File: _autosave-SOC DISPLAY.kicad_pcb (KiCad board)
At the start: 2 copper layers, 44.7 x 50.3 mm, 87 parts, among them IC101 LM5164QDDATQ1, IC501 CM BLE, J201 PRG, J202 Conn_01x05_Socket, J203 OLED, J204 OLED, J205 Conn_01x02_Socket, J601 Conn_01x02_Pin, J602 Conn_01x02_Pin, Q301 NDT3055L, U101 TPS563200, U102 LP2985-3.3, U201 STM32G0B1CBTx, U202 MAX485E, U401 TJA1051T-3, U601 INA228AQDGSRQ1

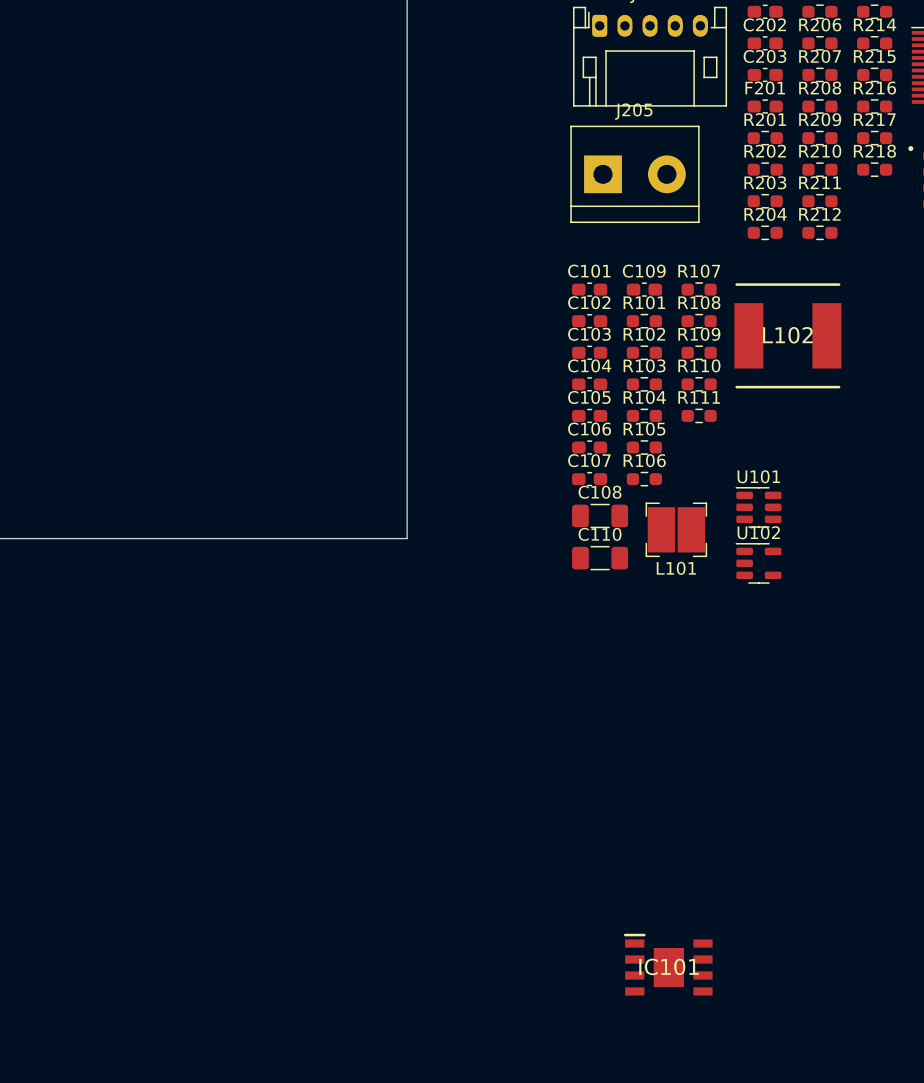
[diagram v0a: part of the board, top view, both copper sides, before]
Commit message: New
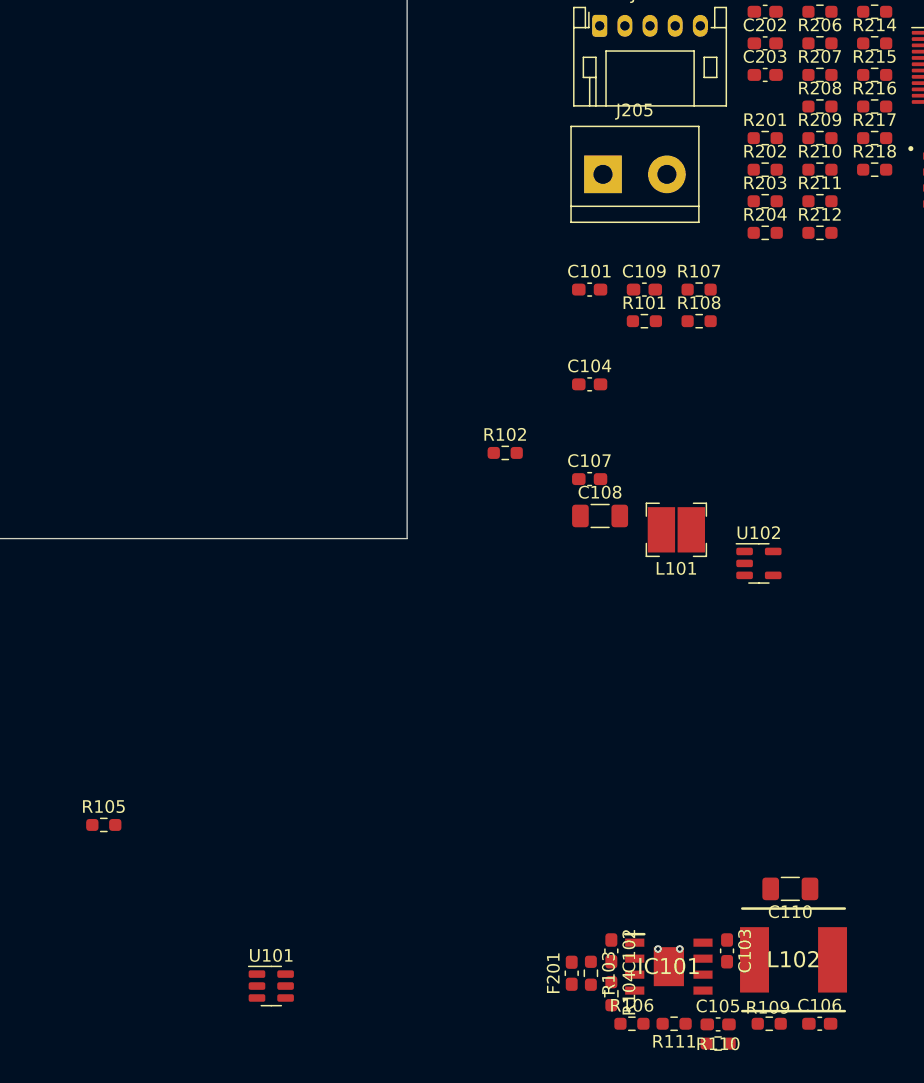
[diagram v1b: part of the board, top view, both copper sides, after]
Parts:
- C101: value 0.1uf -> 22uf
- moved F201 70.6 mm to (87.9, 117.9), turned to 90 degrees
- moved U101 54.3 mm to (64.0, 118.9)
- moved R109 53.6 mm to (103.6, 121.9)
- moved R110 52.4 mm to (99.5, 123.4), turned to 180 degrees
- moved R105 52.4 mm to (50.7, 106.1)
- moved C102 50.1 mm to (91.0, 116.1), turned to -90 degrees
- moved L102 49.6 mm to (105.5, 116.8)
- moved C105 49.4 mm to (99.5, 121.9)
- moved C106 49.3 mm to (107.6, 121.9)
- moved C103 48.8 mm to (100.2, 116.1), turned to -90 degrees
- moved R111 48.3 mm to (96.0, 121.9), turned to 180 degrees
- moved R103 47.0 mm to (89.4, 117.9), turned to -90 degrees
- moved R104 46.0 mm to (91.0, 119.5), turned to -90 degrees
- moved R106 43.3 mm to (92.7, 121.9)
- moved C110 30.3 mm to (105.3, 111.2), turned to 180 degrees
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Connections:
- net Net-(IC101-SW) renamed /POWER_UNIT/sw
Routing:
- net GND: vias 0 -> 2
